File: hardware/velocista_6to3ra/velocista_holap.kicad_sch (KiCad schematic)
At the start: 14 parts, among them J1 ENTRADA, J2 BORNERA_MOTOR_A, J3 BORNERA_MOTOR_B, J5 SENSORES_DE_PISO, SW1 SW_DE_ARRANQUE, U1 LM7805_TO220, U2 INTEGRADO_L293D

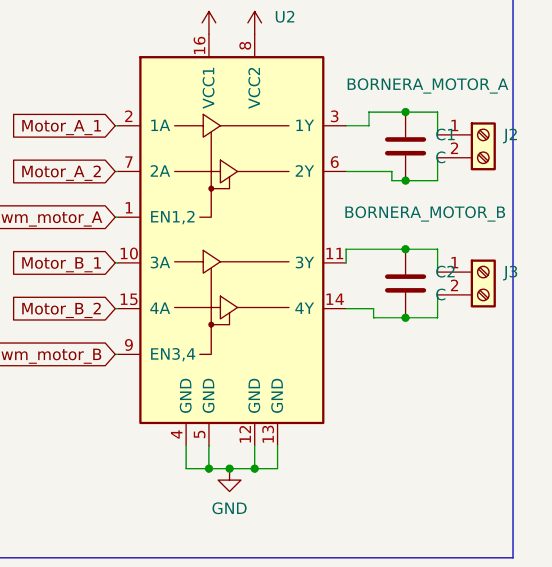
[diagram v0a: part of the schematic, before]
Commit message: 29/10
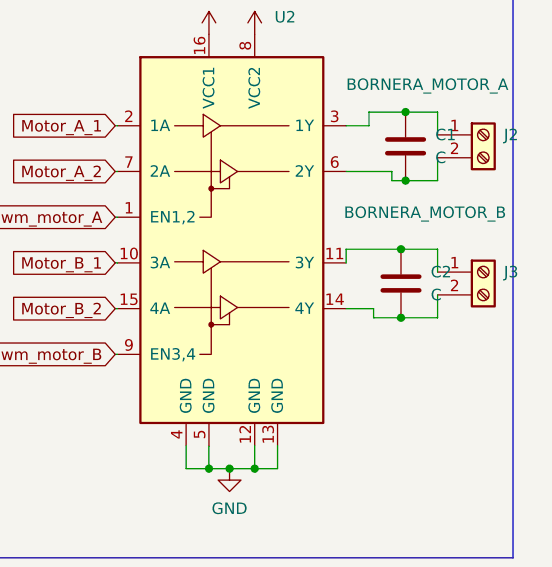
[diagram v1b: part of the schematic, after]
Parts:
- C1, C2: footprint Capacitor_THT:C_Disc_D3.8mm_W2.6mm_P2.50mm -> Capacitor_THT:C_Disc_D4.7mm_W2.5mm_P5.00mm
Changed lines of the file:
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@@
 	)
 	(junction
-		(at 140.208 119.634)
-		(diameter 0)
-		(color 0 0 0 0)
-	)
-	(junction
-		(at 140.208 112.014)
+		(at 139.7 112.014)
 		(diameter 0)
 		(color 0 0 0 0)
@@
 	)
 	(junction
+		(at 139.7 119.634)
+		(diameter 0)
+		(color 0 0 0 0)
+	)
+	(junction
 		(at 59.944 38.354)
 		(diameter 0)
@@
 	(wire
 		(pts
+			(xy 139.7 119.634) (xy 143.764 119.634)
+		)
+		(stroke
+			(width 0)
+			(type default)
+		)
+	)
+	(wire
+		(pts
 			(xy 133.604 103.378) (xy 138.684 103.378)
 		)
@@
 	(wire
 		(pts
-			(xy 136.652 119.634) (xy 140.208 119.634)
+			(xy 136.652 119.634) (xy 139.7 119.634)
 		)
 		(stroke
@@
 	(wire
 		(pts
-			(xy 143.764 119.634) (xy 140.208 119.634)
-		)
-		(stroke
-			(width 0)
-			(type default)
-		)
-	)
-	(wire
-		(pts
 			(xy 115.824 133.858) (xy 115.824 136.398)
 		)
@@
 	(wire
 		(pts
-			(xy 140.208 112.014) (xy 133.604 112.014)
+			(xy 133.604 112.014) (xy 139.7 112.014)
 		)
 		(stroke
@@
 	(wire
 		(pts
+			(xy 139.7 112.014) (xy 143.764 112.014)
+		)
+		(stroke
+			(width 0)
+			(type default)
+		)
+	)
+	(wire
+		(pts
 			(xy 108.204 108.458) (xy 107.95 108.458)
 		)
@@
 		(pts
 			(xy 138.684 103.378) (xy 138.684 104.394)
-		)
-		(stroke
-			(width 0)
-			(type default)
-		)
-	)
-	(wire
-		(pts
-			(xy 143.764 112.014) (xy 140.208 112.014)
 		)
 		(stroke
@@
 			)
 		)
-		(property "Footprint" "Capacitor_THT:C_Disc_D3.8mm_W2.6mm_P2.50mm"
+		(property "Footprint" "Capacitor_THT:C_Disc_D4.7mm_W2.5mm_P5.00mm"
 			(at 141.1732 104.394 0)
 			(effects
@@
 	)
 	(symbol
-		(lib_id "Device:C")
-		(at 140.208 115.824 0)
-		(unit 1)
-		(exclude_from_sim no)
-		(in_bom yes)
-		(on_board yes)
-		(dnp no)
-		(fields_autoplaced yes)
-		(property "Reference" "C2"
-			(at 143.51 114.5539 0)
-			(effects
-				(font
-					(size 1.27 1.27)
-				)
-				(justify left)
-			)
-		)
-		(property "Value" "C"
-			(at 143.51 117.0939 0)
-			(effects
-				(font
-					(size 1.27 1.27)
-				)
-				(justify left)
-			)
-		)
-		(property "Footprint" "Capacitor_THT:C_Disc_D3.8mm_W2.6mm_P2.50mm"
-			(at 141.1732 119.634 0)
-			(effects
-				(font
-					(size 1.27 1.27)
-				)
-				(hide yes)
-			)
-		)
-		(property "Datasheet" "~"
-			(at 140.208 115.824 0)
-			(effects
-				(font
-					(size 1.27 1.27)
-				)
-				(hide yes)
-			)
-		)
-		(property "Description" "Unpolarized capacitor"
-			(at 140.208 115.824 0)
-			(effects
-				(font
-					(size 1.27 1.27)
-				)
-				(hide yes)
-			)
-		)
-		(pin "1"
-		)
-		(pin "2"
-		)
-		(instances
-			(project "velocista_holap"
-				(path "/1010dc30-9ded-4f78-9883-94d6f7871a3f"
-					(reference "C2")
-					(unit 1)
-				)
-			)
-		)
-	)
-	(symbol
 		(lib_id "Regulator_Linear:LM7805_TO220")
 		(at 74.422 38.354 0)
@@
 					(unit 1)
 				)
+			)
+		)
+	)
+	(symbol
+		(lib_id "Device:C")
+		(at 139.7 115.824 0)
+		(unit 1)
+		(exclude_from_sim no)
+		(in_bom yes)
+		(on_board yes)
+		(dnp no)
+		(fields_autoplaced yes)
+		(property "Reference" "C2"
+			(at 143.002 114.5539 0)
+			(effects
+				(font
+					(size 1.27 1.27)
+				)
+				(justify left)
+			)
+		)
+		(property "Value" "C"
+			(at 143.002 117.0939 0)
+			(effects
+				(font
+					(size 1.27 1.27)
+				)
+				(justify left)
+			)
+		)
+		(property "Footprint" "Capacitor_THT:C_Disc_D4.7mm_W2.5mm_P5.00mm"
+			(at 140.6652 119.634 0)
+			(effects
+				(font
+					(size 1.27 1.27)
+				)
+				(hide yes)
+			)
+		)
+		(property "Datasheet" "~"
+			(at 139.7 115.824 0)
+			(effects
+				(font
+					(size 1.27 1.27)
+				)
+				(hide yes)
+			)
+		)
+		(property "Description" "Unpolarized capacitor"
+			(at 139.7 115.824 0)
+			(effects
+				(font
+					(size 1.27 1.27)
+				)
+				(hide yes)
+			)
+		)
+		(pin "1"
+		)
+		(pin "2"
+		)
+		(instances
+			(project "velocista_holap"
+				(path "/1010dc30-9ded-4f78-9883-94d6f7871a3f"
+					(reference "C2")
+					(unit 1)
+				)

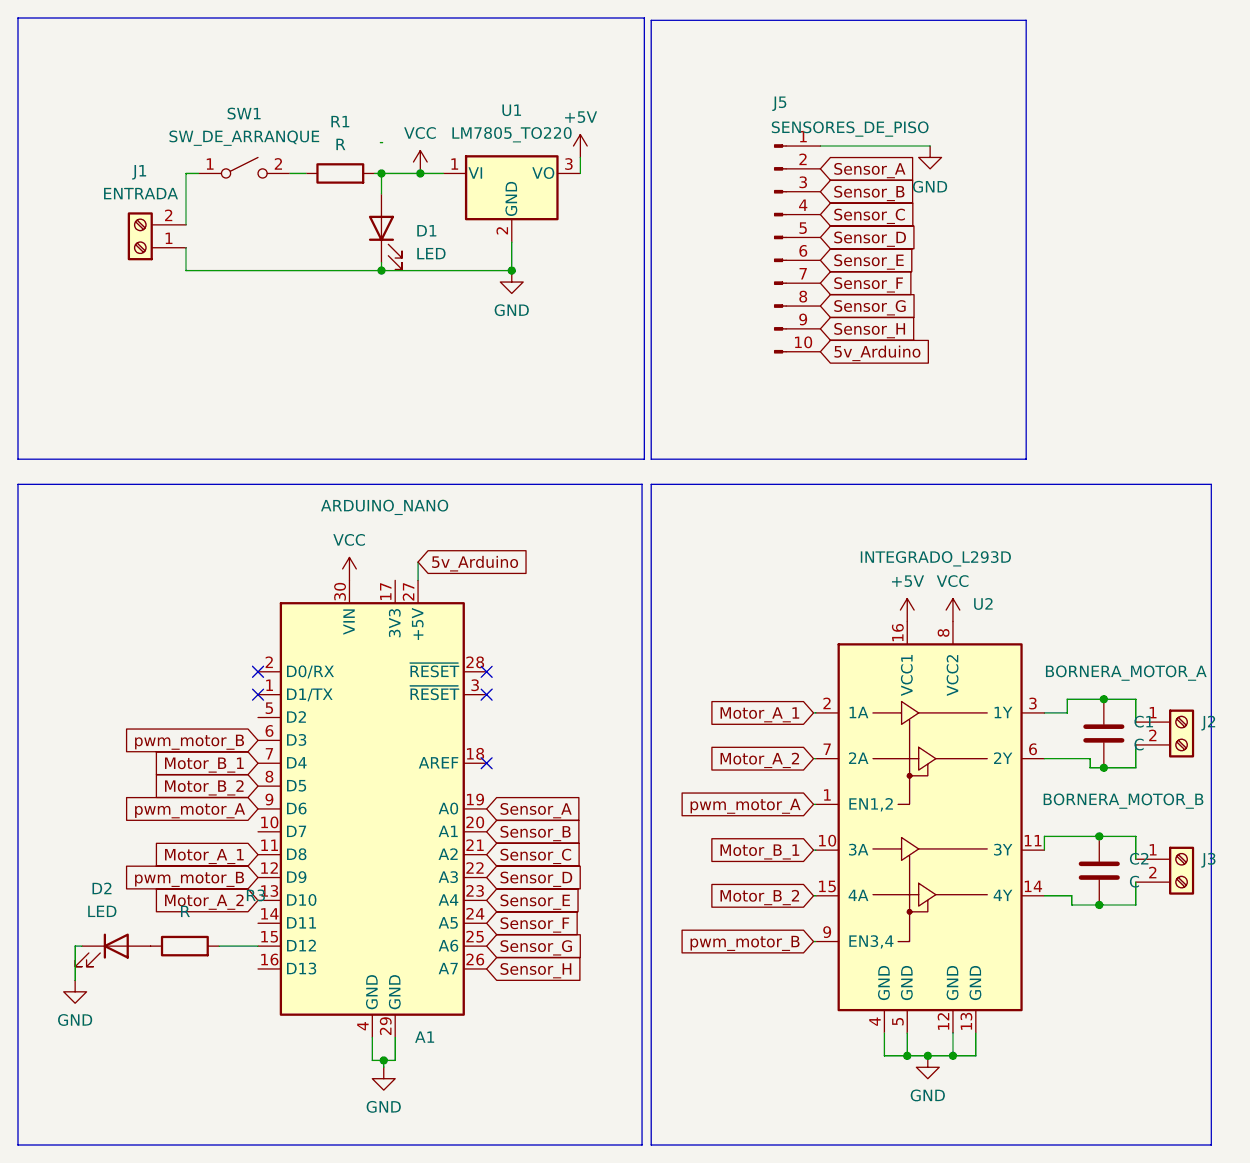
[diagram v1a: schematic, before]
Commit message: 29/10_2
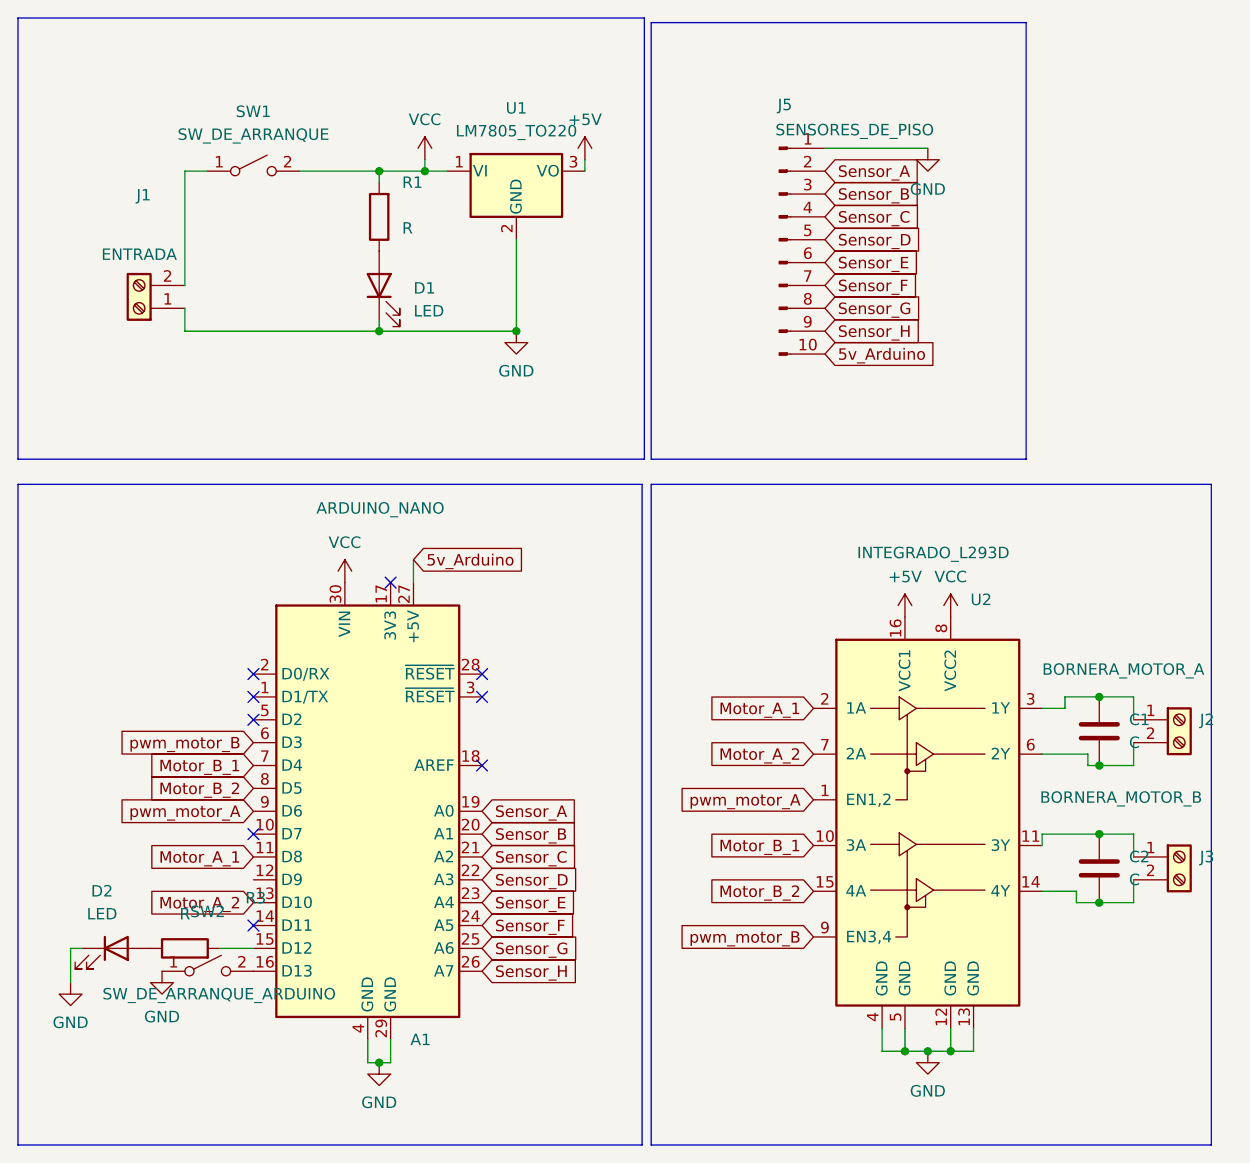
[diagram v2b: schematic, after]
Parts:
- added SW2: SW_DE_ARRANQUE_ARDUINO, Button_Switch_THT:SW_Tactile_Straight_KSA0Axx1LFTR, symbol Switch:SW_SPST
- U1: footprint Package_TO_SOT_THT:TO-220-3_Vertical -> EESTN5:TO-220-2
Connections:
- net GND: now also SW2.1 (A)
- net VCC: now also SW1.2 (B); no longer D1.2 (A)
- net pwm_motor_B: no longer A1.12 (D9)
- net at A1.16 (D13): now also SW2.2 (B)
- net at R1.1: now also D1.2 (A); no longer SW1.2 (B)
- no-connect marks 5 -> 9
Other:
- moved on the sheet: A1, C1, D1, J1, J5, R1, SW1, U1, U2
